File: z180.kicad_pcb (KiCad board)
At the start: 2 copper layers, 89.7 x 64.8 mm, 69 parts, among them J1 SERIAL_IO, J2 USB_POWER, J3 zdbus, J4 zabus, J5 zcbus, J6 USB_DATA, J7 POWER_IN, J8 Conn_01x08, J9 MEM_ADDR, SW1 SW_Push, U1 74LS138, U2 28C256, U3 AS6C1008-55PCN, U4 74LS138, U5 DS1813, U8 74LS05, Y1 Crystal

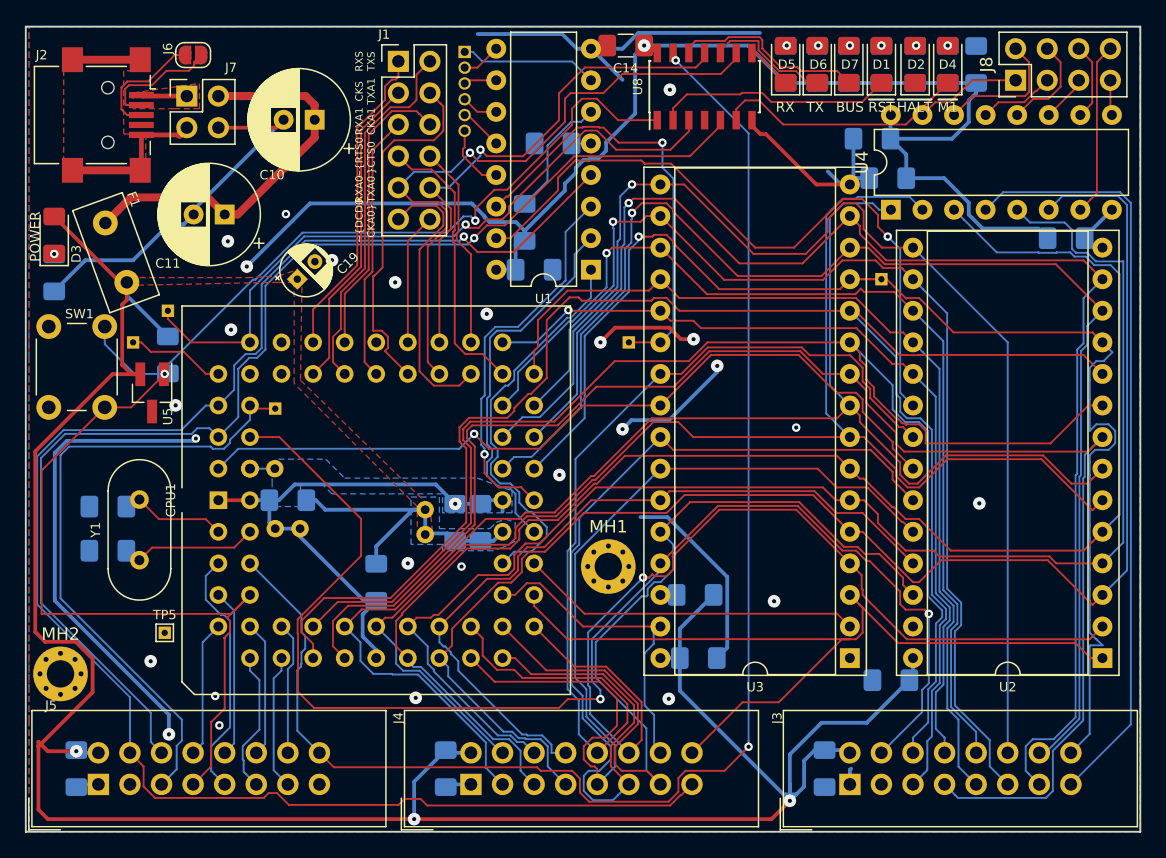
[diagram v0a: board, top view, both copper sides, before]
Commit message: layout mostly complete
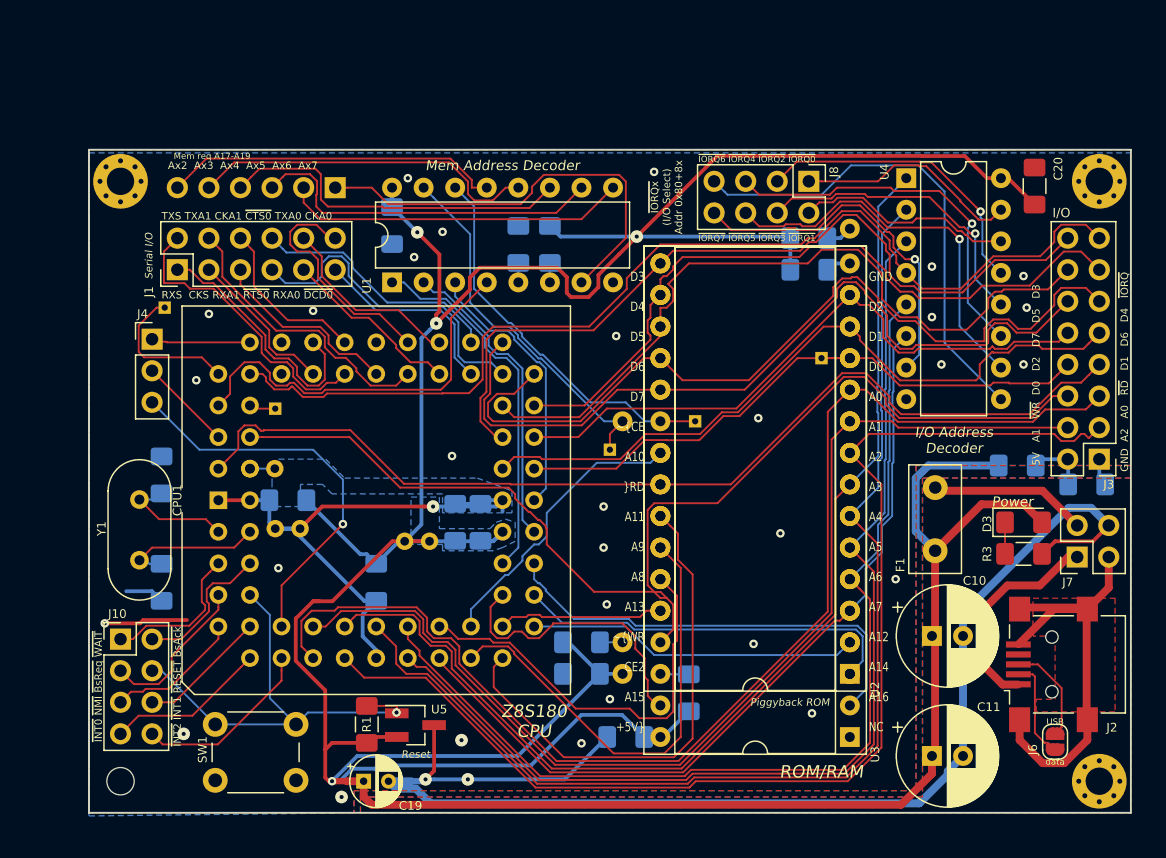
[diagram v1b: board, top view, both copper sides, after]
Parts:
- removed C14, C17, C7, C8: 0.1µF, Capacitor_SMD:C_1206_3216Metric_Pad1.42x1.75mm_HandSolder
- removed D1, D2, D4, D5, D6, D7: LED, LED_SMD:LED_1206_3216Metric_Pad1.42x1.75mm_HandSolder
- removed J5: zcbus, Connector_IDC:IDC-Header_2x08_P2.54mm_Vertical
- removed R5, R6, R7, R8: 300, Resistor_SMD:R_1206_3216Metric_Pad1.42x1.75mm_HandSolder
- removed TP5: TST_WAIT, TestPoint:TestPoint_THTPad_1.0x1.0mm_Drill0.5mm
- removed TP6: TST_HALT, TestPoint:TestPoint_THTPad_1.0x1.0mm_Drill0.5mm
- removed U8: 74LS05, Package_SO:SOIC-14_3.9x8.7mm_P1.27mm
- added J10: BUSCTRL, Connector_PinHeader_2.54mm:PinHeader_2x04_P2.54mm_Vertical, F.Cu at (48.3, 141.0)
- added JP1: SolderJumper_2_Bridged, NetTie:NetTie-2_SMD_Pad0.5mm, F.Cu at (66.0, 152.4)
- added JP2: SolderJumper_2_Bridged, NetTie:NetTie-2_SMD_Pad0.5mm, B.Cu at (72.1, 152.4)
- added MH3: MountingHole_Pad, MountingHole:MountingHole_2.2mm_M2_Pad_Via, F.Cu at (48.3, 104.1)
- added MH4: MountingHole_Pad, MountingHole:MountingHole_2.2mm_M2_Pad_Via, F.Cu at (127.0, 104.1)
- C20: value C_Small -> 0.1µF; moved to F.Cu
- J3: footprint Connector_IDC:IDC-Header_2x08_P2.54mm_Vertical -> Connector_PinHeader_2.54mm:PinHeader_2x08_P2.54mm_Vertical
- J4: value zabus -> STATUS; footprint Connector_IDC:IDC-Header_2x08_P2.54mm_Vertical -> Connector_PinHeader_2.54mm:PinHeader_1x03_P2.54mm_Vertical
- J9: footprint Connector_PinHeader_1.27mm:PinHeader_1x06_P1.27mm_Vertical -> Connector_PinHeader_2.54mm:PinHeader_1x06_P2.54mm_Vertical
- MH2: footprint MountingHole:MountingHole_2.2mm_M2_Pad_Via -> MountingHole:MountingHole_2.2mm_M2
- R1, R3: moved to F.Cu
- R2: value 300 -> 10k
- R4: value 300 -> 22R
- U2: footprint Package_DIP:DIP-28_W15.24mm_Socket -> z180:DIP-28_Piggyback_Memory_W15.24mm_Socket
- moved J6 88.7 mm to (123.4, 149.2), turned to 270 degrees
- moved J2 87.9 mm to (123.2, 143.0), turned to 90 degrees
- moved C9 84.4 mm to (126.0, 128.5), turned to 0 degrees
- moved D3 81.3 mm to (120.9, 131.6), turned to 0 degrees
- moved R3 81.2 mm to (120.9, 134.1), turned to 0 degrees
- moved J7 80.7 mm to (125.2, 134.4), turned to 90 degrees
- moved C11 71.7 mm to (113.5, 150.4), turned to 0 degrees
- moved F1 68.5 mm to (113.8, 133.9), turned to 90 degrees
- moved C10 64.7 mm to (113.5, 140.7), turned to 0 degrees
- moved R2 52.4 mm to (85.3, 141.2), turned to 0 degrees
- moved J4 44.1 mm to (50.8, 116.8), turned to 0 degrees
- moved MH1 43.1 mm to (127.0, 152.4)
- moved C19 40.7 mm to (67.8, 152.4), turned to 0 degrees
- moved U5 34.1 mm to (72.0, 147.9), turned to 0 degrees
- moved R1 33.8 mm to (68.1, 147.8), turned to 270 degrees
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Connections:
- net Net-(R10-Pad2) renamed /G1
- net Net-(R11-Pad1) renamed /~G2B
- net Net-(R9-Pad2) renamed /CE2
- C10 pad 1: /PWRIN_5V -> /REG_5V
- C10 pad 2: Earth -> /PWRIN_GND
- C11 pad 1: /PWRIN_5V -> /REG_5V
- C11 pad 2: Earth -> /PWRIN_GND
- C19 pad 1: +5V -> /REG_5V
- C19 pad 2: Earth -> /PWRIN_GND
- C9 pad 1: +5V -> /IO_5V
- D3 pad 2: +5V -> /REG_5V
- F1 pad 1: +5V -> /REG_5V
- J3 pad 10: /D5 -> /D2
- J3 pad 11: /D4 -> /D6
- J3 pad 12: /D3 -> /D7
- J3 pad 13: /D2 -> /D4
- J3 pad 14: /D1 -> /D5
- J3 pad 16: /D0 -> /D3
- J3 pad 2: +5V -> /IO_5V
- J3 pad 3: /~RD -> /A2
- J3 pad 4: /~WR -> /A1
- J3 pad 6: /A1 -> /~WR
- J3 pad 7: /A2 -> /~RD
- J3 pad 8: /D7 -> /D0
- J3 pad 9: /D6 -> /D1
- J4 pad 1: Earth -> /~HALT
- J4 pad 2: +5V -> /~M1
- J4 pad 3: /A3 -> /ST
- J7 pad 4: Earth -> /PWRIN_GND
- MH1 pad 1: Earth -> /PWRIN_GND
- R2 pad 2: Net-(D1-Pad2) -> /~EEWR
- R3 pad 2: Earth -> /PWRIN_GND
- R4 pad 1: +5V -> /REG_5V
- R4 pad 2: Net-(D2-Pad2) -> /IO_5V
- U2 pad 27: Net-(U2-Pad27) -> /~EEWR
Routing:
- net Earth: track 203.7 -> 84.5 mm, vias 26 -> 33
- net /~BUSACK: track 115.8 -> 11.7 mm, vias 2 -> 0
- net /~MREQ: track 135.5 -> 32.0 mm, vias 1 -> 0
- net +5V: track 328.3 -> 231.9 mm, vias 5 -> 4
- net /~M1: track 99.8 -> 7.54 mm, vias 1 -> 0
- net /REG_5V: track 0.00 -> 92.0 mm
- net /PWRIN_GND: track 0.00 -> 84.1 mm
- net /~RESET: track 118.9 -> 37.9 mm, vias 2 -> 1
- net /A13: track 74.2 -> 13.4 mm
- net /D2: track 111.1 -> 51.3 mm, vias 1 -> 0
- net /A10: track 80.7 -> 23.2 mm
- net /D0: track 107.0 -> 50.6 mm, vias 1 -> 0
- net /A7: track 120.7 -> 66.4 mm
- net /A12: track 78.6 -> 26.8 mm, vias 1 -> 0
- net /D1: track 107.4 -> 57.3 mm, vias 1 -> 0
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- added copper zone on B.Cu, net /PWRIN_GND
- added copper zone on F.Cu, net /PWRIN_GND
- removed copper zone on F.Cu, net +5V
- removed copper zone on F.Cu, net /USB_Vbus
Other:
- board size 89.7 x 64.8 mm -> 83.8 x 53.3 mm
- board text added: "+"
- board text added: "-"
- board text added: "1"
- board text added: "5V A1 ~WR~ D0 D2 D7 D5 D3"
- board text added: "A10 A8 A6 A4 A3 A1 ST ~INT1~ ~NMI~"
- board text added: "A9 A7 A5 GND A2 A0 ~INT2~ ~INT0~"
- board text added: "Ax2 Ax3 Ax4 Ax5 Ax6 Ax7"
- board text added: "D3 D4 D5 D6 D7 ~CE A10 ~RD A11 A9 A8 A13 ~WR CE2 A15 +5V"
- board text added: "D7 D6 D4 D5 D2 D3 D0 D1 A19 GND A18 +5V A16 A17 A14 A15 A12 A13 A11"
- board text added: "GND A2 A0 ~RD~ D1 D6 D4 ~IORQ~"
- board text added: "GND D2 D1 D0 A0 A1 A2 A3 A4 A5 A6 A7 A12 A14 A16 NC"
- board text added: "I/O"
- board text added: "I/O Address Decoder"
- board text added: "Mem Address Decoder"
- board text added: "Piggyback ROM"
- board text added: "Power"
- board text added: "ROM/RAM"
- board text added: "RXS CKS RXA1 ~RTS0~ RXA0 ~DCD0~"
- board text added: "Reset"
- board text added: "Serial I/O"
- board text added: "TXS TXA1 CKA1 ~CTS0~ TXA0 CKA0"
- board text added: "USB data"
- board text added: "Z8S180 CPU"
- board text added: "~CTS0~ TXA0 CKA0 NC ~CKA1~ RXS ~DREQ1~ ~HALT~"
- board text added: "~INT0~ ~NMI~ ~BsReq~ ~WAIT~"
- board text added: "~INT2~ ~INT1~ ~RESET~ ~BsAck~"
- board text added: "~IORQ6~ ~IORQ4~ ~IORQ2~ ~IORQ0~"
- board text added: "~IORQ7~ ~IORQ5~ ~IORQ3~ ~IORQ1~"
- board text added: "~IORQx~ (I/O Select) Addr 0x80+8x"
- board text added: "~IORQ~ ~RFSH~ E ~MREQ~ ~WR~ ~M1~ PHI ~RD~ GND GND EXTAL XTAL ~BUSACK~ ~WAIT~ ~RESET~ ~BUSREQ~"
- board text added: "~RTS0~ ~DCD0~ RXA0 TXA1 RXA1 TXS CKS TEND1"
- board text removed: "7 6 5 4 3 2"
- board text removed: "A13 A11 A9 A7 A5 A3 GND"
- board text removed: "A14 A15 A12 A10 A8 A6 A4 5V"
- board text removed: "BUS"
- board text removed: "CKS TXA1"
- board text removed: "D0 D1 D3 D5 D7 A1 ~WR~ 5V"
- board text removed: "POWER"
- board text removed: "RX"
- board text removed: "RXA0 TXA0"
- board text removed: "RXA1 CKA1"
- board text removed: "RXS TXS"
- board text removed: "ST"
- board text removed: "TX"
- board text removed: "~BUS ACK"
- board text removed: "~BUS REQ"
- board text removed: "~DCD0 CKA0"
- board text removed: "~HALT"
- board text removed: "~INT0"
- board text removed: "~INT1"
- board text removed: "~INT2"
- board text removed: "~IORQ~ D2 D4 D6 A2 A0 ~RD~ GND"
- board text removed: "~M1"
- board text removed: "~MREQ"
- board text removed: "~NMI"
- board text removed: "~RST"
- board text removed: "~RTS0 ~CTS0"
- board text removed: "~WAIT"
